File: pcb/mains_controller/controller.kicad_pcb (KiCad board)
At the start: 2 copper layers, 60 x 70 mm, 27 parts, among them J1 Conn_01x03, J2 Conn_01x03, J6 MFRC_CONN, J7 Micro_SD_Card, J8 Conn_01x03, J9 Conn_01x03, Q3 IRLL014N, U3 W25Q32JVSS

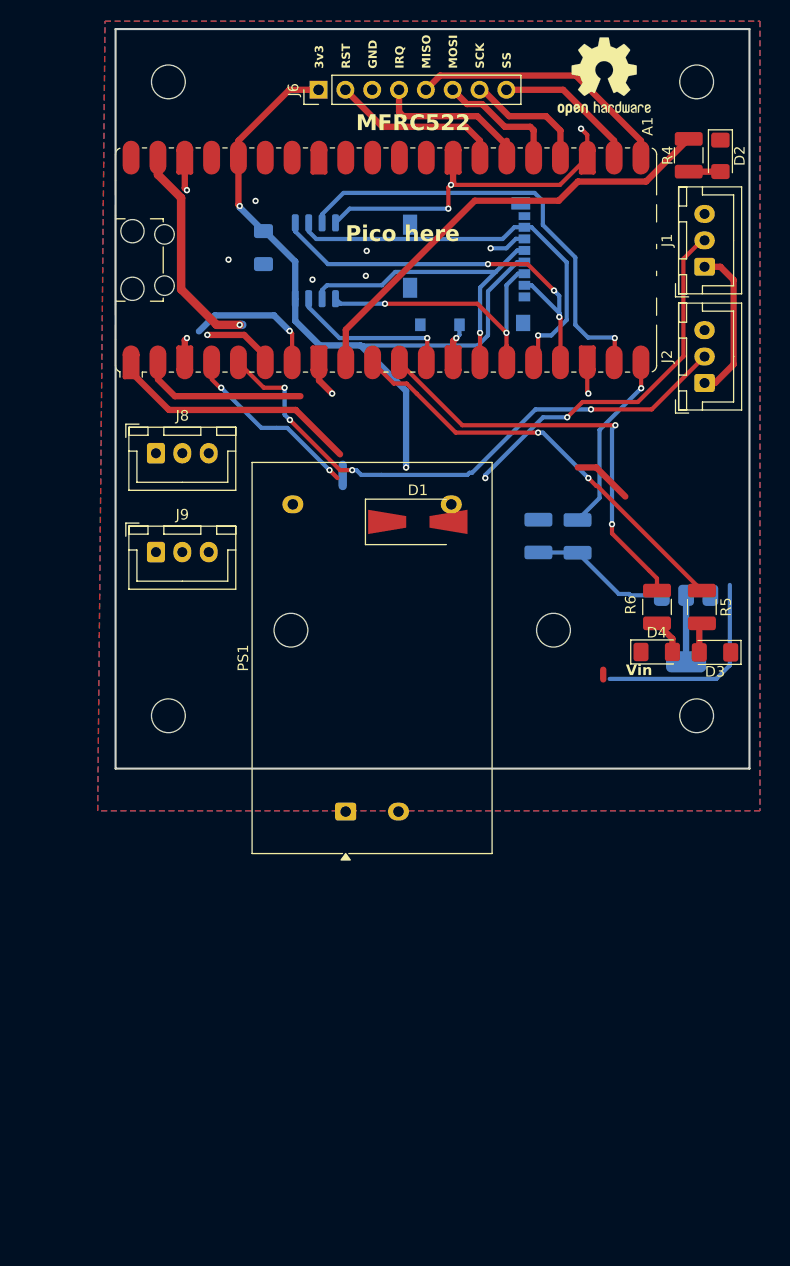
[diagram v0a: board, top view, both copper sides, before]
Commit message: Production version (sent to JLC!)
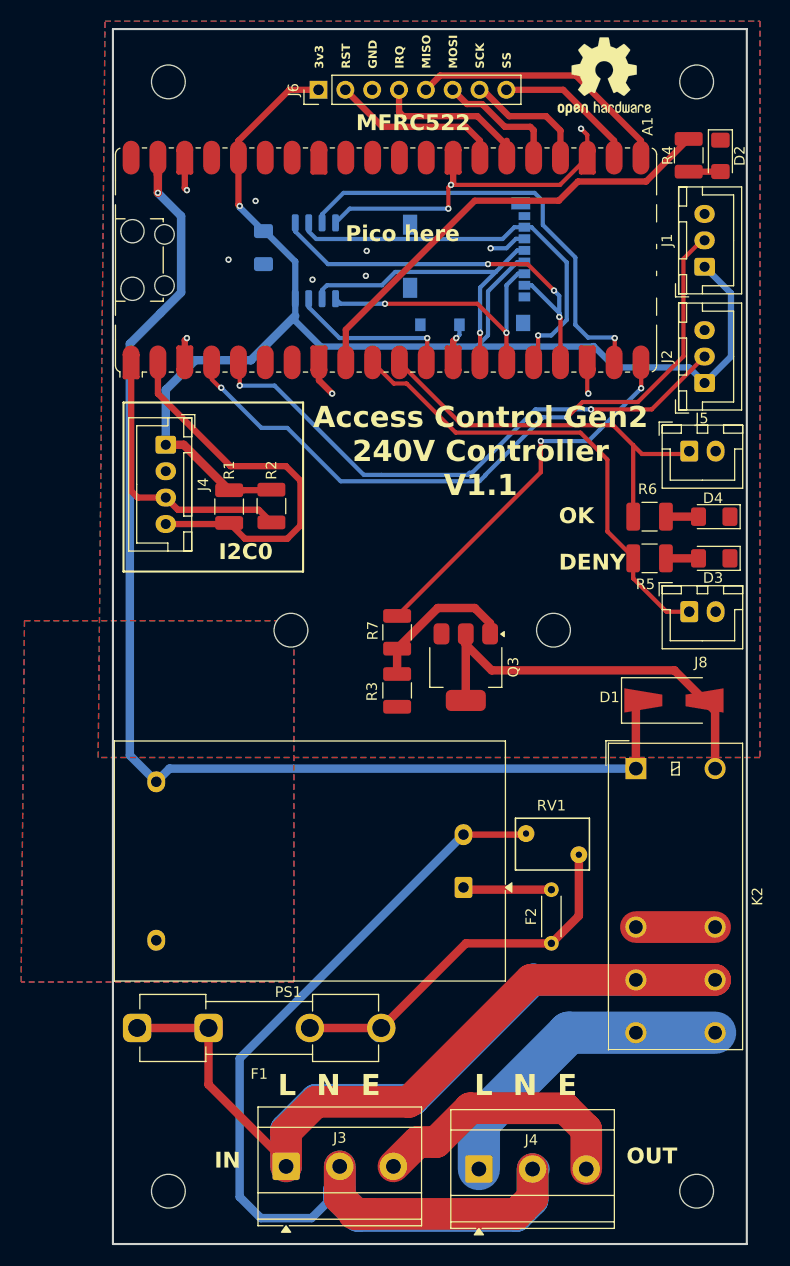
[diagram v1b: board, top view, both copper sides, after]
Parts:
- removed J9: Conn_01x03, Connector_JST:JST_XH_B3B-XH-A_1x03_P2.50mm_Vertical
- added F1: Fuse, Fuse:Fuseholder_Clip-5x20mm_Keystone_3517_Inline_P23.11x6.76mm_D1.70mm_Horizontal, F.Cu at (33.3, 112.8)
- added F2: Fuse, Resistor_THT:R_Axial_DIN0204_L3.6mm_D1.6mm_P5.08mm_Horizontal, F.Cu at (72.5, 104.8)
- added J3: Conn_01x03, TerminalBlock_MetzConnect:TerminalBlock_MetzConnect_Type073_RT02603HBLU_1x03_P5.08mm_Horizontal, F.Cu at (47.4, 125.9)
- added J4: Conn_01x04_Pin, Connector_JST:JST_XH_B4B-XH-A_1x04_P2.50mm_Vertical, F.Cu at (36.0, 57.6)
- added J4: Conn_01x03, TerminalBlock_MetzConnect:TerminalBlock_MetzConnect_Type073_RT02603HBLU_1x03_P5.08mm_Horizontal, F.Cu at (65.6, 126.2)
- added J5: Conn_01x02_Pin, Connector_JST:JST_XH_B2B-XH-A_1x02_P2.50mm_Vertical, F.Cu at (85.5, 58.2)
- added K2: Relay_SPDT, Relay_THT:Relay_SPDT_Omron_G2RL-1-E, F.Cu at (80.5, 88.2)
- added R1: 4k7, Resistor_SMD:R_1210_3225Metric_Pad1.30x2.65mm_HandSolder, F.Cu at (42.0, 63.5)
- added R2: 4k7, Resistor_SMD:R_1210_3225Metric_Pad1.30x2.65mm_HandSolder, F.Cu at (46.0, 63.4)
- added RV1: Varistor, Varistor:RV_Disc_D7mm_W4.9mm_P5mm, F.Cu at (75.1, 96.4)
- J8: value Conn_01x03 -> Conn_01x02_Pin; footprint Connector_JST:JST_XH_B3B-XH-A_1x03_P2.50mm_Vertical -> Connector_JST:JST_XH_B2B-XH-A_1x02_P2.50mm_Vertical
- Q3, R3, R7: moved to F.Cu
- moved J8 52.7 mm to (85.5, 73.4)
- moved REF** 45.0 mm to (36.2, 128.2)
- moved REF** 45.0 mm to (86.2, 128.2)
- moved D1 29.5 mm to (84.1, 81.8)
- moved Q3 21.2 mm to (64.4, 78.7)
- moved R3 19.8 mm to (57.9, 80.8), turned to -90 degrees
- moved R7 19.3 mm to (57.9, 75.3)
- moved D4 13.9 mm to (87.9, 64.4), turned to 180 degrees
- moved PS1 13.3 mm to (64.2, 99.5), turned to 180 degrees
- moved D3 8.90 mm to (87.9, 68.3)
- moved R6 8.57 mm to (81.8, 64.4), turned to 0 degrees
- moved R5 6.76 mm to (81.8, 68.3), turned to 0 degrees
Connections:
- A1 pad 1: RS485_TX -> I2C0_SDA
- A1 pad 2: RS485_RX -> I2C0_SCL
- J8 pad 1: +3V3 -> ACCESS_GRANTED
- J8 pad 2: GPIO_ACC3 -> GND
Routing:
- net LINE: track 0.00 -> 129.9 mm
- net NEUT: track 0.00 -> 113.3 mm
- net RELAY+: track 23.8 -> 117.7 mm
- net I2C0_SCL: track 0.00 -> 38.5 mm
- net Net-(F1-Pad2): track 0.00 -> 37.3 mm
- net RELAY-: track 6.30 -> 39.0 mm
- net SW_LINE: track 0.00 -> 30.3 mm
- net I2C0_SDA: track 0.00 -> 26.7 mm
- net Earth: track 0.00 -> 25.1 mm
- net RS485_TX: track 23.9 -> 0.00 mm
- net MOSFET_GATE: track 17.4 -> 36.2 mm, vias 1 -> 2
- net RS485_RX: track 15.8 -> 0.00 mm
- net GPIO_ACC1: track 52.1 -> 66.2 mm, vias 4 -> 2
- net GPIO_ACC4: track 13.2 -> 0.30 mm, vias 1 -> 0
- net +3V3: track 120.9 -> 132.2 mm, vias 2 -> 1
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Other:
- board size 60 x 70 mm -> 60 x 115 mm
- board text added: "+"
- board text added: "+3v3 GND SDA SCL"
- board text added: "Access Control Gen2 240V Controller V1.1"
- board text added: "DENY"
- board text added: "I2C0"
- board text added: "IN"
- board text added: "L N E"
- board text added: "OK"
- board text added: "OUT"
- board text removed: "Access Control Gen2 LowVolt Controller V1.1"
- board text removed: "GP4"
- board text removed: "Relay Mosfet"
- board text removed: "Vin"
